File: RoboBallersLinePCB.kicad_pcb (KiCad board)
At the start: 2 copper layers, 132 x 132 mm, 116 parts, among them J2 Bottom PCB, Q1 P-Channel, Q2 N-Channel, U1 MCP3008, U2 MCP3008, U3 MCP3008, U4 BoostConverter, U5 NSL-32, U6 NSL-32, U7 Solenoid-Electric

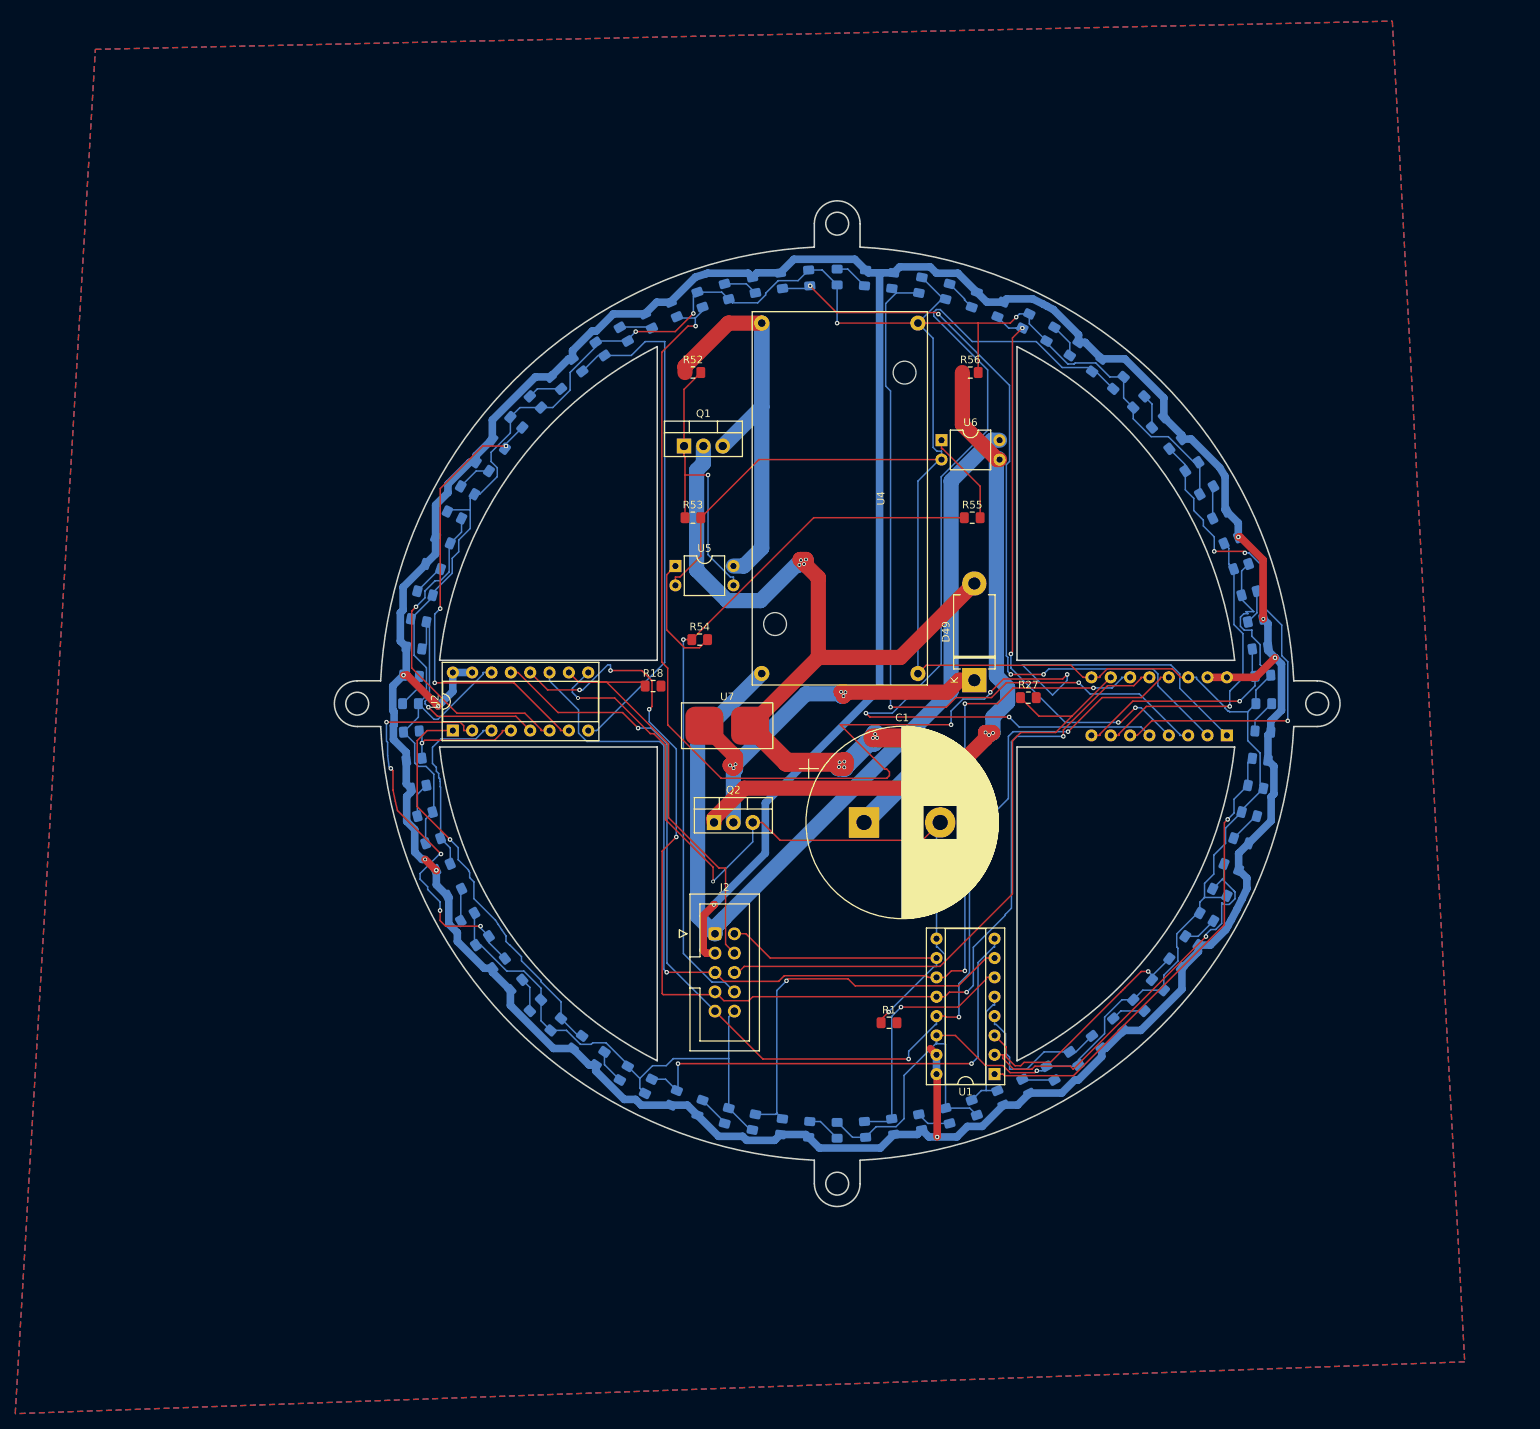
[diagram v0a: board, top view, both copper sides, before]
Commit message: redid whole pcb
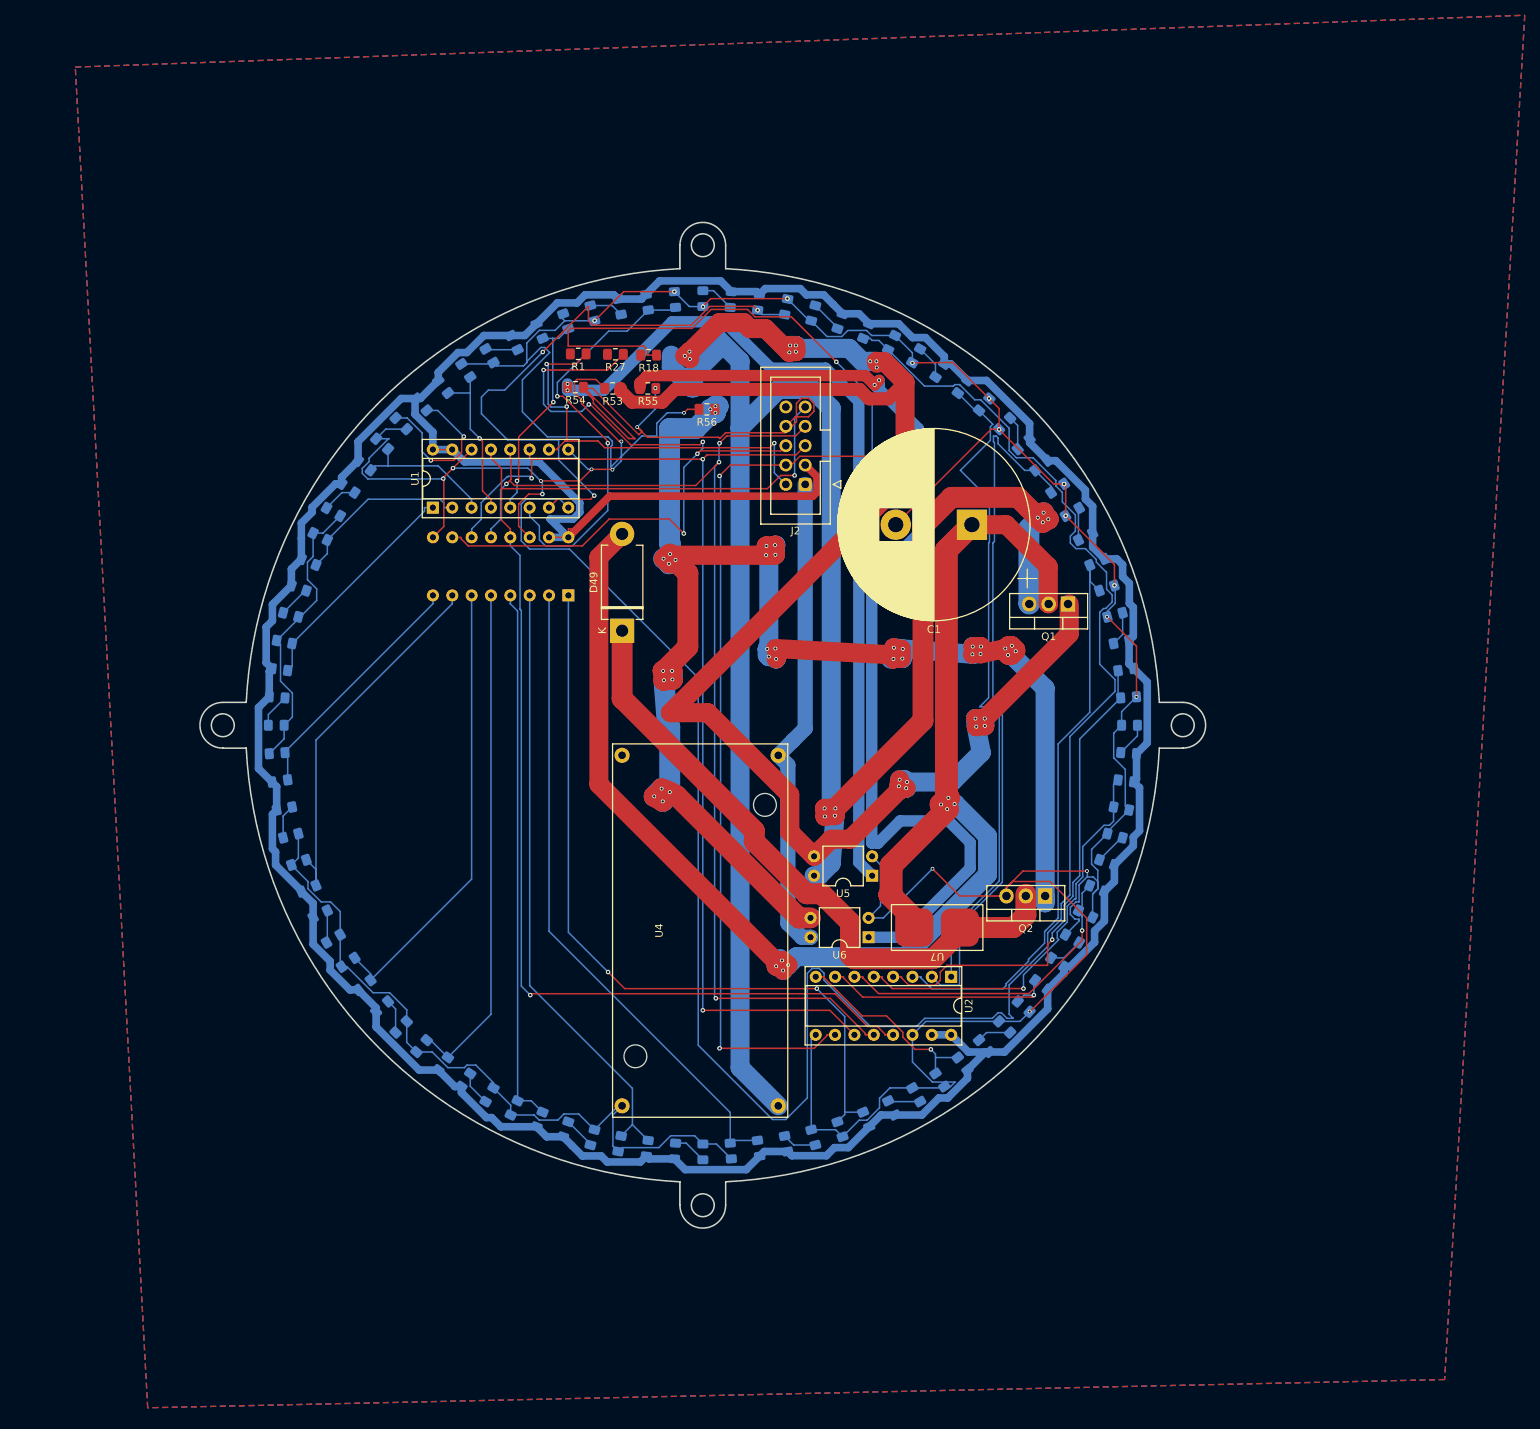
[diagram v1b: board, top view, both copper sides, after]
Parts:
- R52: moved to B.Cu
- moved D48 129.8 mm to (226.9, 310.1), turned to -172 degrees
- moved R26 129.8 mm to (227.5, 313.8), turned to -169 degrees
- moved R51 129.8 mm to (226.5, 306.5), turned to -176 degrees
- moved D24 129.8 mm to (228.3, 317.3), turned to -165 degrees
- moved D1 129.7 mm to (226.4, 302.8), turned to 180 degrees
- moved R50 129.6 mm to (229.4, 320.8), turned to -161 degrees
- moved R2 129.5 mm to (226.5, 299.2), turned to 176 degrees
- moved D47 129.4 mm to (230.6, 324.3), turned to -157 degrees
- moved D25 129.2 mm to (226.9, 295.5), turned to 173 degrees
- moved R25 129.2 mm to (232.2, 327.6), turned to -154 degrees
- moved R28 128.9 mm to (227.5, 291.9), turned to 169 degrees
- moved D23 128.8 mm to (233.9, 330.8), turned to -150 degrees
- moved D2 128.5 mm to (228.3, 288.3), turned to 165 degrees
- moved R49 128.4 mm to (235.8, 333.9), turned to -146 degrees
- moved R3 128.0 mm to (229.4, 284.8), turned to 161 degrees
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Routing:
- net 48v: track 65.7 -> 278.3 mm, vias 0 -> 8
- net CH71: track 63.7 -> 276.0 mm, vias 2 -> 0
- net Net-(Q1-G): track 39.2 -> 230.9 mm, vias 1 -> 18
- net Net-(Q2-G): track 96.2 -> 251.4 mm, vias 3 -> 35
- net Net-(U6-A): track 12.3 -> 141.5 mm, vias 0 -> 2
- net CSLS2: track 55.8 -> 180.9 mm, vias 0 -> 4
- net Net-(U5-A): track 15.6 -> 110.5 mm, vias 0 -> 2
- net GND: track 687.4 -> 609.7 mm, vias 7 -> 23
- net CH03: track 176.7 -> 101.7 mm, vias 4 -> 2
- net CH43: track 130.1 -> 66.7 mm, vias 2 -> 0
- net Net-(D49-K): track 138.2 -> 195.4 mm, vias 15 -> 8
- net 12v: track 121.1 -> 67.2 mm
- net CH22: track 25.0 -> 76.8 mm
- net CH32: track 16.2 -> 65.0 mm
- net CH72: track 67.5 -> 25.8 mm, vias 0 -> 1
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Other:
- outline, holes or cut-outs redrawn
